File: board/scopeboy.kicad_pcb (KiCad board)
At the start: 4 copper layers, 100 x 80 mm, 151 parts, among them J1 USB_C_Receptacle_USB2.0_16P, J2 SM03B-SRSS-TB, J3 SM03B-SRSS-TB, J4 Conn_01x10, J5 SM04B-SRSS-TB, J6 HDMI_A, J7 731000105, J8 Conn_01x02, J9 Conn_01x08, SW1 SW_Push, SW2 SW_Push, SW3 RotaryEncoder_Switch, U1 W25Q128JVS, U10 LMH6629, U11 OPA820, U12 DAC5571, U13 LM4040DBZ-2.0, U14 TLV3501, U15 DAC5571, U16 TLV9101, U17 TLV62568DBVR, U18 MT3608 (TPS61023DRLR), U2 DNF, U4 RP2350_80QFN, U5 TPS2116DRL, U6 LM27762, U7 ADC08060, U8 OPA354, U9 ADG621, Y1 ABM8-272-T3

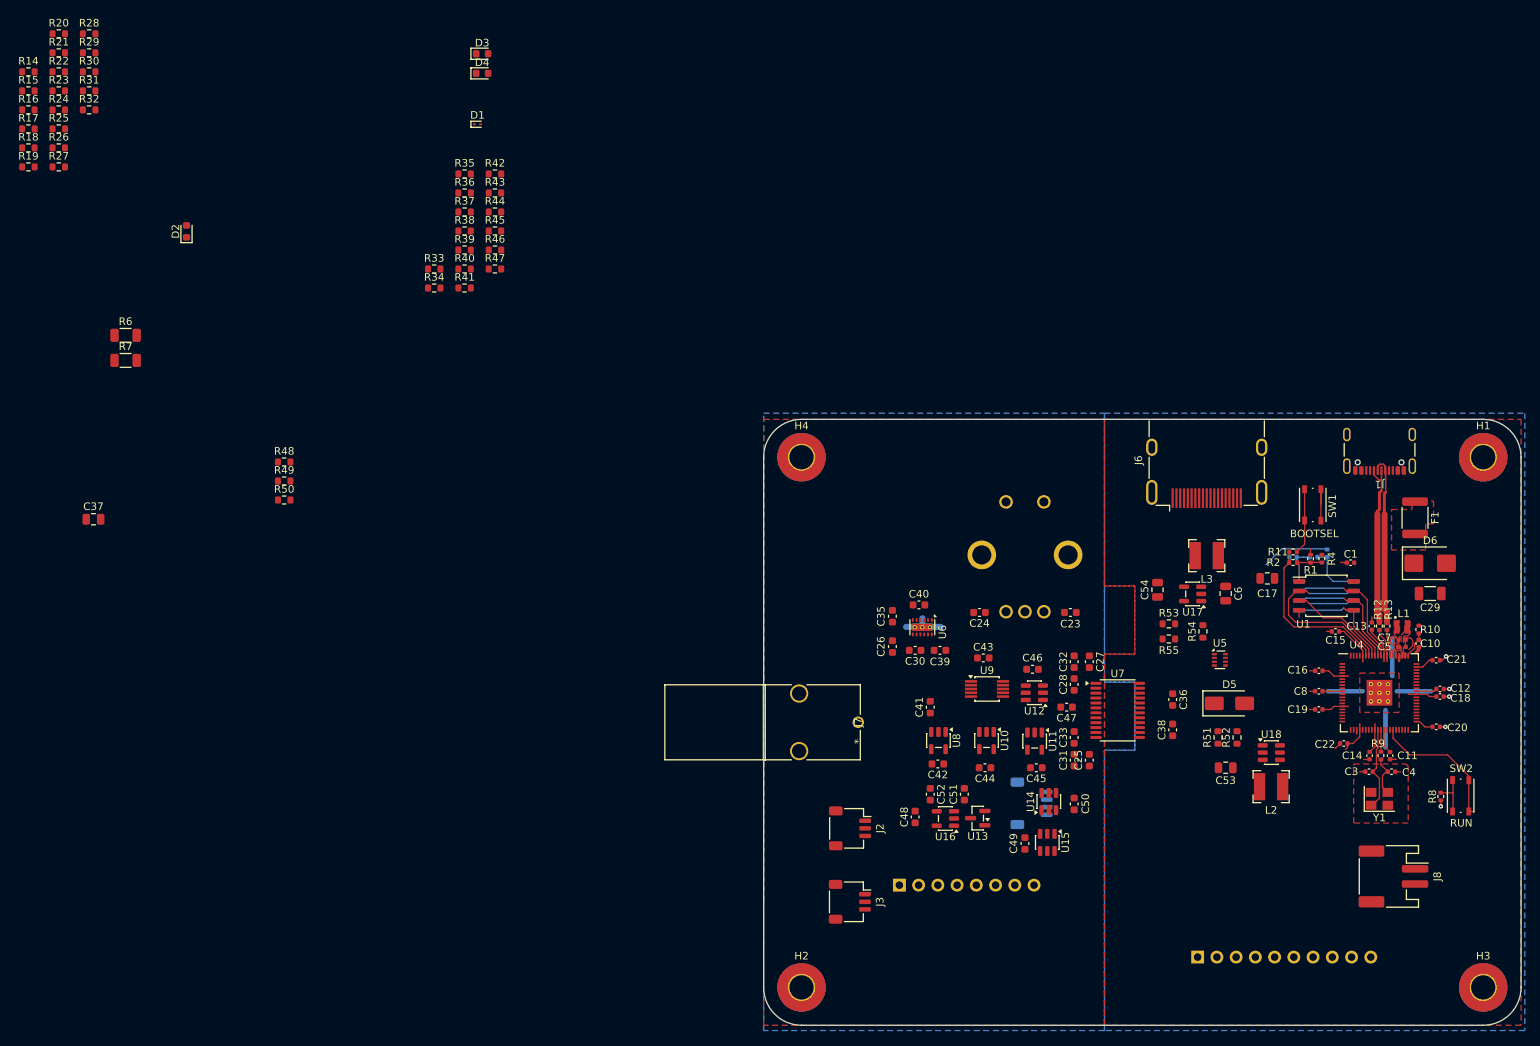
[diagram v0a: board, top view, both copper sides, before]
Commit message: Production version of board
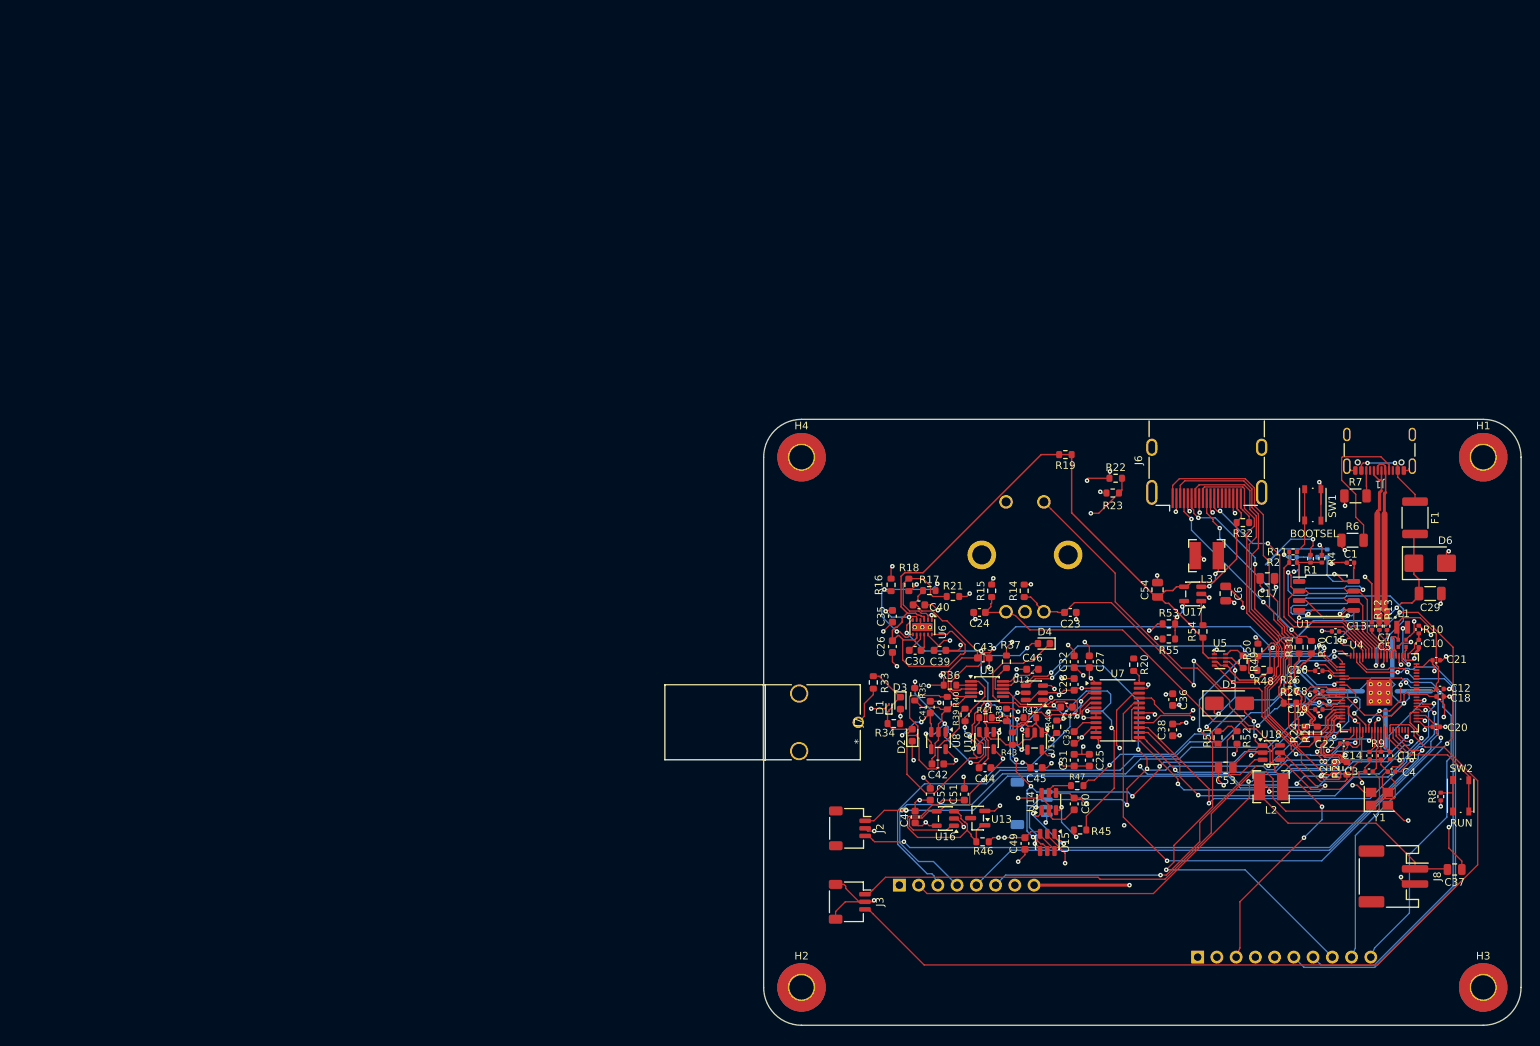
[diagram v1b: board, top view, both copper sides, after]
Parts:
- moved R29 191.1 mm to (197.7, 115.9), turned to 90 degrees
- moved R28 190.9 mm to (196.0, 115.9), turned to 90 degrees
- moved C37 185.6 mm to (211.9, 129.3), turned to 180 degrees
- moved R25 184.3 mm to (193.8, 111.3), turned to 90 degrees
- moved R24 184.0 mm to (192.1, 111.3), turned to 90 degrees
- moved R30 178.4 mm to (193.0, 99.9), turned to -90 degrees
- moved R26 177.7 mm to (190.1, 105.7)
- moved R27 177.3 mm to (190.1, 107.3)
- moved R31 175.8 mm to (191.3, 99.9), turned to -90 degrees
- moved R20 164.6 mm to (169.5, 102.2), turned to -90 degrees
- moved R6 164.2 mm to (198.4, 85.8)
- moved R7 163.4 mm to (198.8, 80.0)
- moved R32 161.8 mm to (183.9, 83.5), turned to 180 degrees
- moved R22 149.5 mm to (167.1, 77.6)
- moved R23 148.9 mm to (166.7, 79.6)
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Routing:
- net GND: track 20.4 -> 272.2 mm, vias 5 -> 56
- net VDC: track 0.00 -> 125.3 mm
- net /SWD: track 0.00 -> 116.3 mm
- net -3V3: track 0.00 -> 101.6 mm, vias 0 -> 5
- net /SWCLK: track 0.00 -> 94.5 mm
- net +3.3V: track 43.7 -> 133.3 mm, vias 0 -> 26
- net /SD_D0: track 0.00 -> 88.8 mm, vias 0 -> 1
- net GNDA: track 5.72 -> 93.1 mm, vias 0 -> 32
- net /TX: track 0.00 -> 84.8 mm, vias 0 -> 2
- net /SCL: track 0.00 -> 82.7 mm, vias 0 -> 6
- net /CSSD: track 0.00 -> 80.9 mm, vias 0 -> 1
- net /DISD: track 0.00 -> 80.7 mm, vias 0 -> 1
- net /RX: track 0.00 -> 80.5 mm, vias 0 -> 2
- net /MISO: track 0.28 -> 75.5 mm, vias 0 -> 3
- net /D2: track 0.00 -> 72.8 mm, vias 0 -> 2
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- added copper zone on In2.Cu, net +3.3VA
- added copper zone on In1.Cu, net GND
- removed copper zone on F.Cu, net +1V1
- removed copper zone on F.Cu, net +3.3V
- removed copper zone on In2.Cu, net -3V3
- removed copper zone on F.Cu, net /VREG_LX
- removed copper zone on B.Cu, net GND
- removed copper zone on F.Cu, net GND
- removed copper zone on B.Cu, net GNDA
- removed copper zone on F.Cu, net GNDA
- removed copper zone on F.Cu, net VBUS
- removed copper zone on In2.Cu, net VBUS
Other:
- rule pad_to_mask_clearance: 0.03 -> 0
